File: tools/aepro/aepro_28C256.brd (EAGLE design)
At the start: 53 x 80 mm, 23 parts, among them IC1 MCP23017SP, IC2 MCP23008/P, U1 328P, Y1 16 MHz

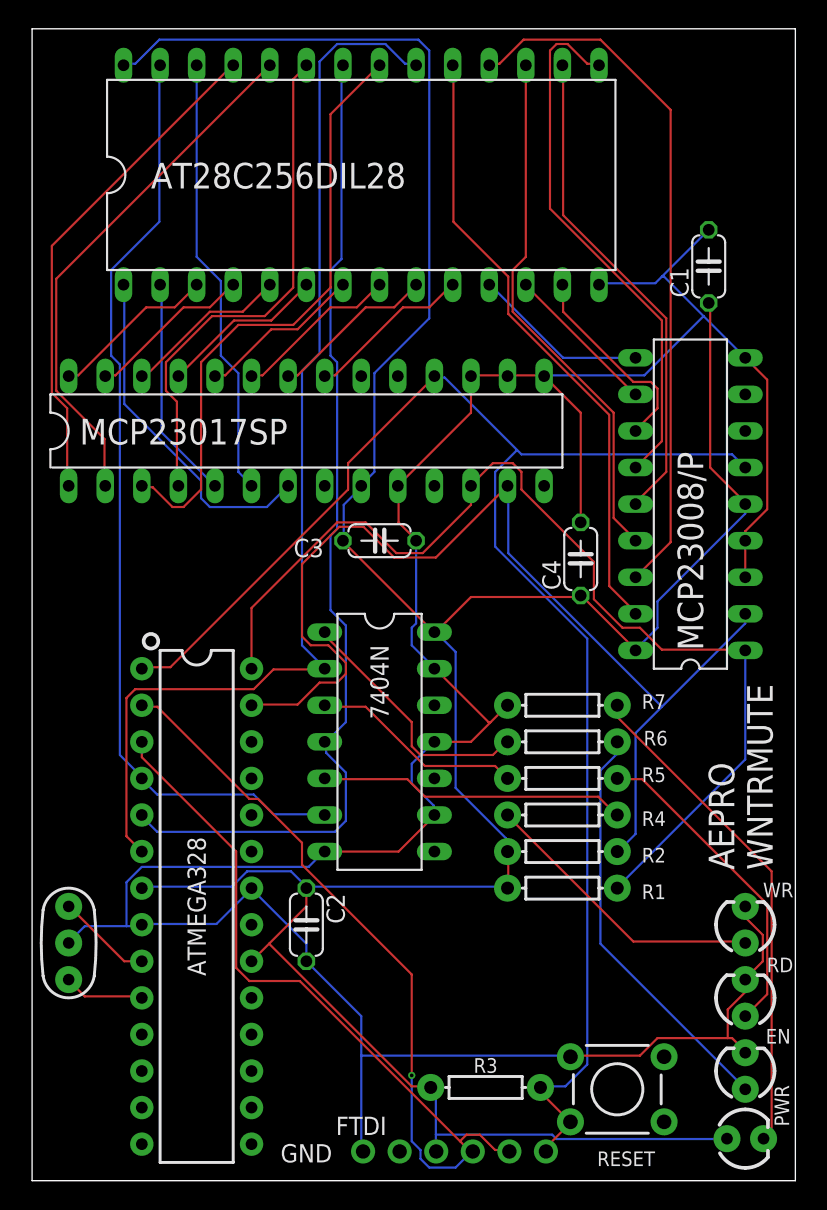
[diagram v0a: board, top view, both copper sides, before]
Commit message: AEPRO rev 7
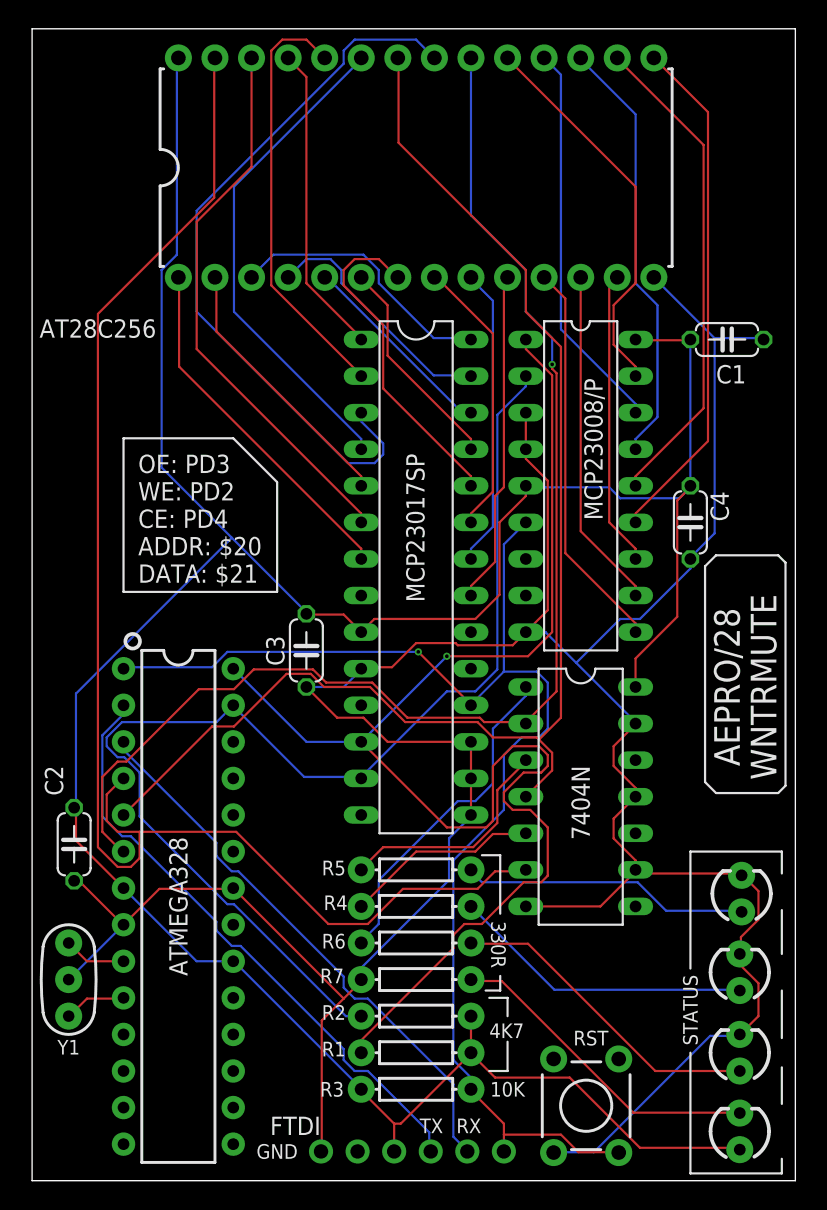
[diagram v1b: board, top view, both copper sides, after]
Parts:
- U$1: value AT28C256DIL28 -> AT28C256; device wntrmute:DIL28-6 -> wntrmute:DIL28-6-ZIF_SOCKET
- moved R7 21.6 mm to (26.7, 14.0)
- moved R6 17.3 mm to (26.7, 16.5)
- moved C2 17.1 mm to (2.92, 23.4)
- moved R1 15.3 mm to (26.7, 8.89), turned to 0 degrees
- moved R2 15.3 mm to (26.7, 11.4), turned to 0 degrees
- moved V1 14.5 mm to (38.1, 26.7)
- moved IC1 12.7 mm to (26.7, 41.9), turned to 270 degrees
- moved R5 12.0 mm to (26.7, 21.6)
- moved R4 12.0 mm to (26.7, 19.1), turned to 0 degrees
- moved C3 9.16 mm to (19.1, 36.8), turned to 270 degrees
- moved C4 8.03 mm to (45.7, 45.7), turned to 270 degrees
- moved IC2 7.73 mm to (38.1, 48.3), turned to 270 degrees
- moved D3 7.24 mm to (49.3, 19.9)
- moved C1 5.24 mm to (48.3, 58.4), turned to 0 degrees
- moved R3 4.83 mm to (26.7, 6.35)
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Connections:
- net N$2 renamed WE
- net N$3 renamed OE
- net N$4 renamed CE
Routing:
- net WE: track 65.6 -> 100.9 mm
- net SCL: track 73.1 -> 100.1 mm, vias 0 -> 1
- net OE: track 69.9 -> 92.6 mm
- net D6: track 48.8 -> 27.3 mm
- net N$7: track 110.0 -> 89.8 mm, vias 0 -> 1
- net D7: track 43.4 -> 27.0 mm
- net D0: track 12.3 -> 27.3 mm
- net A8: track 35.0 -> 21.7 mm
- net D1: track 10.9 -> 23.7 mm
- net CE: track 76.9 -> 89.4 mm, vias 0 -> 1
- net N$10: track 34.8 -> 22.6 mm
- net A3: track 11.5 -> 23.2 mm
- net A0: track 11.5 -> 23.2 mm
- net GND: track 205.4 -> 214.8 mm
- net A1: track 11.6 -> 20.8 mm
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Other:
- board text added: "10K"
- board text added: "330R"
- board text added: "4K7"
- board text added: "AEPRO/28"
- board text added: "AT28C256"
- board text added: "K_ISOM/OAK_CA"
- board text added: "OE: PD3 WE: PD2 CE: PD4 ADDR: $20 DATA: $21"
- board text added: "REV7/20191010"
- board text added: "RST"
- board text added: "RX"
- board text added: "STATUS"
- board text added: "TX"
- board text added: "WNTRMUTE"
- board text removed: "AEPRO WNTRMUTE"
- board text removed: "EN"
- board text removed: "K_ISOM / OAK_CA REV7/20191002"
- board text removed: "PWR"
- board text removed: "R1/R2: 4K7 R3: 10K ALL OTHER R: 330R C: 0.1µF"
- board text removed: "RD"
- board text removed: "RESET"
- board text removed: "WE: PD2 OE: PD3 CE: PD4 MCP23017: 0x20 MCP23008: 0x21"
- board text removed: "WR"
